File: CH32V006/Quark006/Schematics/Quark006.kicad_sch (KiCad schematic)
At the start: 26 parts, among them J1 ESP32_USB, J10 Conn_01x08, J11 Conn_01x03, J2 WCH_USB, J3 Conn_01x06, J4 Conn_01x02, J5 Conn_01x02, J6 Conn_01x01, J7 Conn_01x01, J8 Conn_01x01, J9 Conn_01x01, SW1 SW_SPST, U1 ESP32-S2-MINI-1U-N4, U2 CH32V003FxPx, U3 TLV1117-33

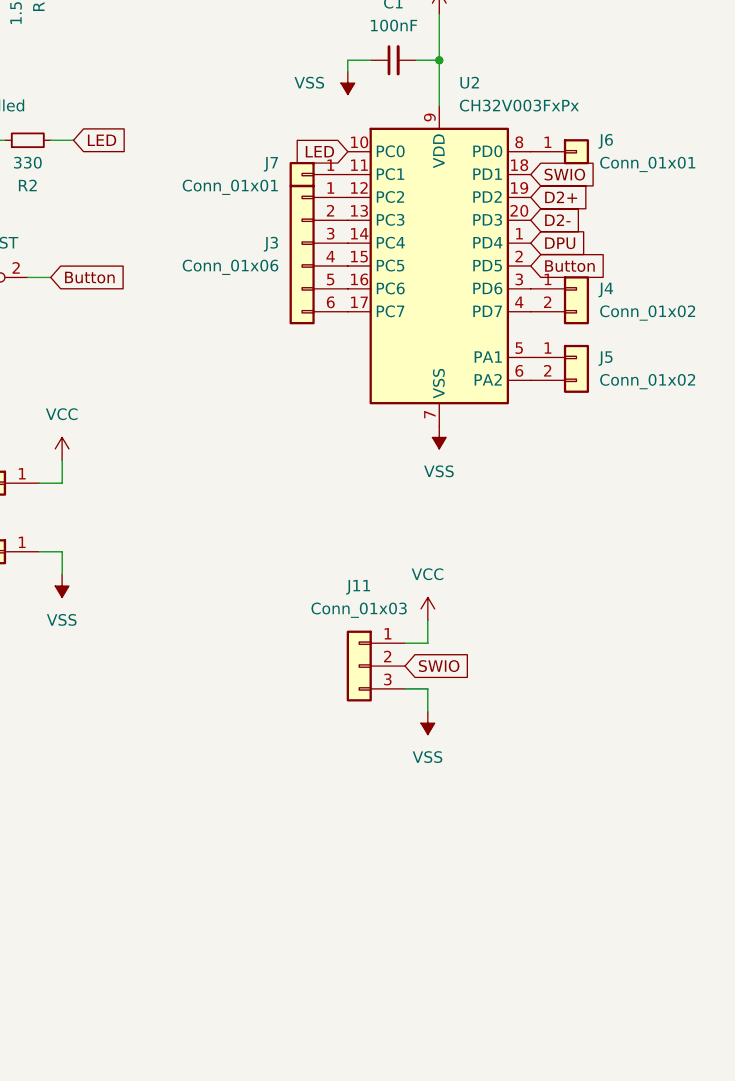
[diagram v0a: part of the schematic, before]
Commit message: moar
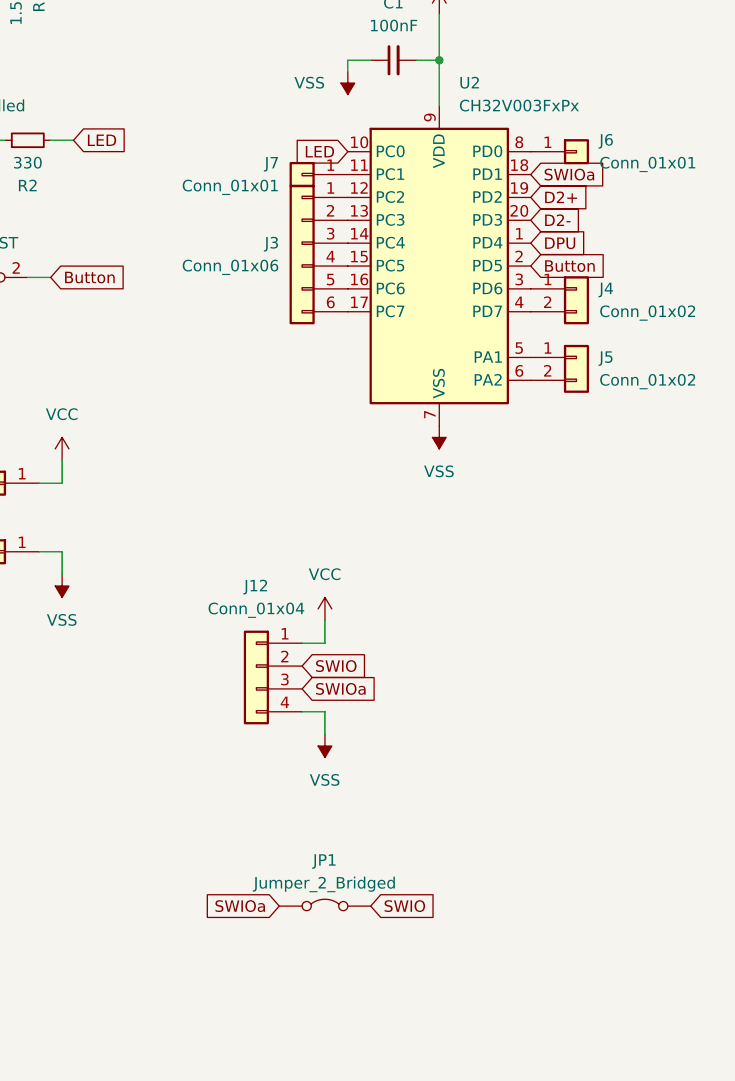
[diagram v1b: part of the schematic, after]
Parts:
- removed J11: Conn_01x03, symbol Connector_Generic:Conn_01x03
- added J12: Conn_01x04, Connector_PinHeader_2.54mm:PinHeader_1x04_P2.54mm_Vertical, symbol Connector_Generic:Conn_01x04
- added JP1: Jumper_2_Bridged, Jumper:SolderJumper-2_P1.3mm_Bridged_RoundedPad1.0x1.5mm, symbol Jumper:Jumper_2_Bridged
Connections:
- net SWIO: now also J12.2 (Pin_2), JP1.2 (B); no longer U2.18 (PD1)
- net VCC: now also J12.1 (Pin_1)
- net VSS: now also J12.4 (Pin_4)
- new net SWIOa: J12.3 (Pin_3), JP1.1 (A), U2.18 (PD1)
